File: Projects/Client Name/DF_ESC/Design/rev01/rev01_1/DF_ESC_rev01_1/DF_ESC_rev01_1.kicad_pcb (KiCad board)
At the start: 4 copper layers, 100 x 75 mm, 187 parts, among them J1 XT60PW-M, J2 HX25003-8AWB, J3 S6B-XH-SM4-TB(LF)(SN), J4 XH-3AWB, J5 7461084, J6 7461084, J7 7461084, J8 USB_C_Receptacle_USB2.0, Q1 HSBA15810C, Q2 HSBA15810C, Q3 HSBA15810C, Q4 HSBA15810C, Q5 HSBA15810C, Q6 HSBA15810C, SW1 SW_DIP_x01, U1 XH-2PWBPZ, U10 PUSB3AB6Z, U2 AMS1117-3.3, U3 STM32F405RGTx, U4 DRV8302DCAR, U5 S4B-XH-SM4-TB-(LF)(SN), U6 ESDCAN24-2BLY, U7 744227S, U8 SN65HVD230, U9 S6B-XH-SM4-TB(LF)(SN), Y1 Crystal_Small

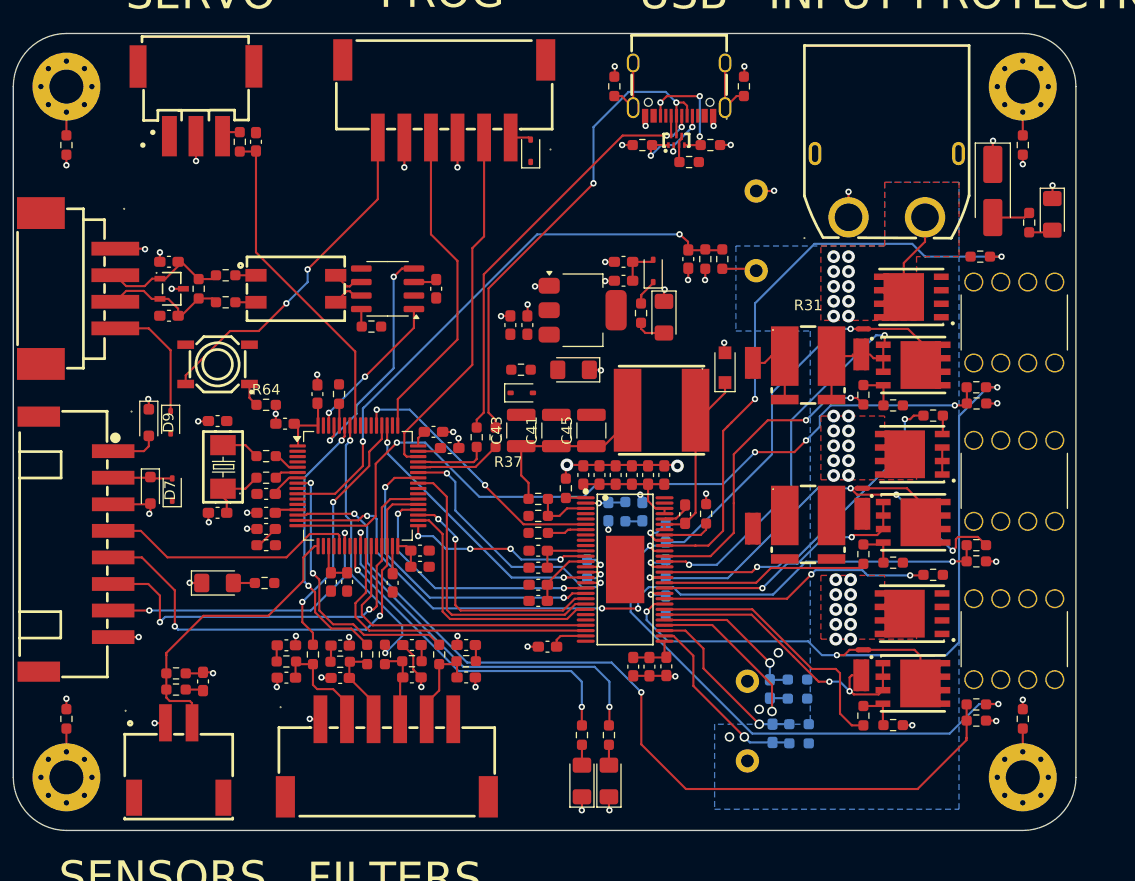
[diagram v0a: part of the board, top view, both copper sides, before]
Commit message: update 20240423
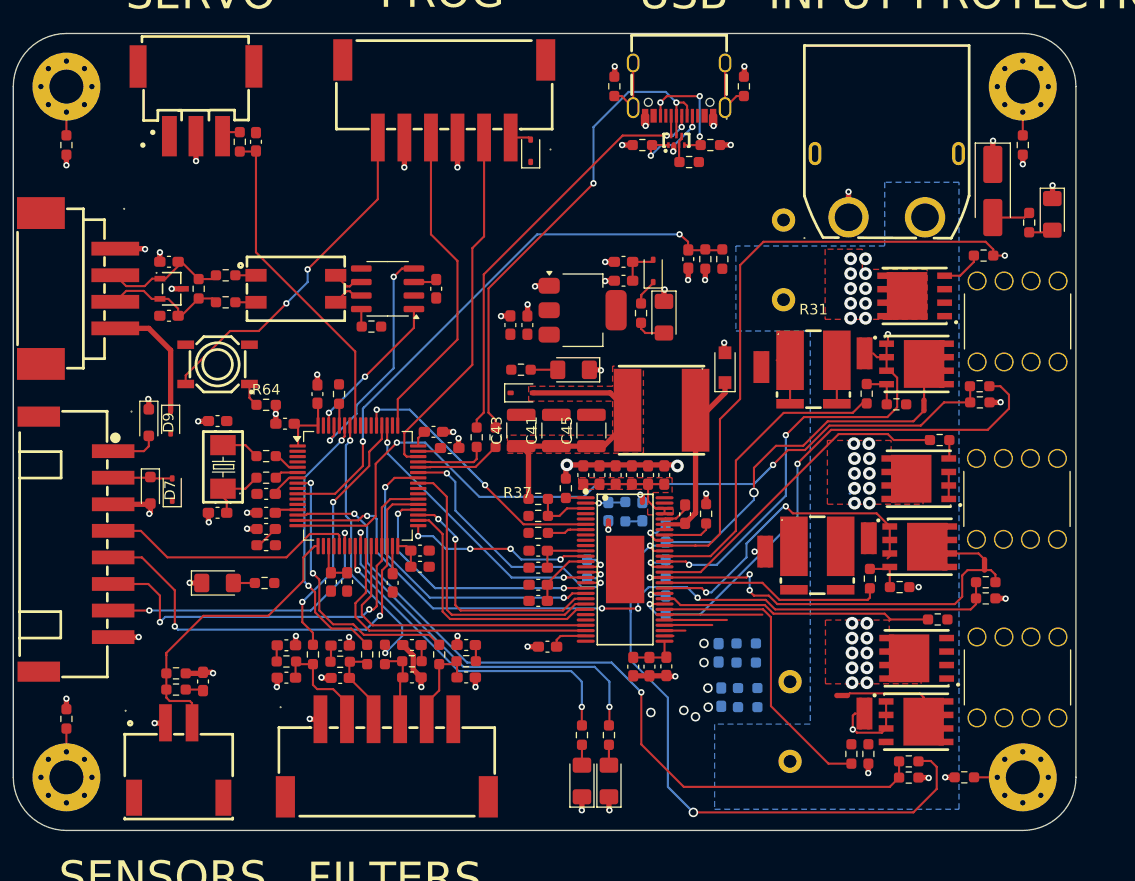
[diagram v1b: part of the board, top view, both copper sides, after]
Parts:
- moved NT4 13.6 mm to (275.2, 146.1), turned to -90 degrees
- moved NT1 9.18 mm to (269.5, 131.1), turned to -90 degrees
- moved R24 8.32 mm to (268.1, 164.6)
- moved R25 8.32 mm to (268.1, 166.1)
- moved R63 7.78 mm to (273.3, 166.1), turned to 180 degrees
- moved C48 5.91 mm to (250.2, 154.4)
- moved C49 5.91 mm to (250.4, 158.6)
- moved R29 5.91 mm to (252.8, 155.3)
- moved R28 5.91 mm to (252.8, 153.5)
- moved R34 5.91 mm to (252.9, 157.7)
- moved R35 5.91 mm to (252.9, 159.5)
- moved NT7 4.74 mm to (261.8, 158.4)
- moved Q5 4.22 mm to (268.8, 154.9)
- moved R39 4.22 mm to (270.8, 151.3)
- moved C1 4.01 mm to (257.0, 162.8)
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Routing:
- net H3_VS: track 72.6 -> 50.2 mm, vias 3 -> 2
- net S2_P: track 17.6 -> 0.84 mm
- net S2_N: track 16.5 -> 1.97 mm
- net S1_P: track 18.0 -> 4.50 mm
- net +VDC: track 31.4 -> 19.9 mm, vias 30 -> 31
- net H3_LOW: track 28.1 -> 16.9 mm, vias 2 -> 1
- net SENS3: track 83.9 -> 74.0 mm
- net /[5] - MOSFET DRIVER/+5V_DRV: track 17.3 -> 26.9 mm
- net H1_VS: track 81.9 -> 91.3 mm
- net S1_N: track 14.9 -> 5.87 mm
- net /[6] - MOSFETs/PHASE_1: track 7.60 -> 3.40 mm
- net /[6] - MOSFETs/PHASE_2: track 9.98 -> 6.05 mm
- net /[6] - MOSFETs/M_H1_RG: track 0.00 -> 3.89 mm
- net H2_LOW: track 25.5 -> 29.4 mm
- net Net-(Q6-G): track 3.97 -> 0.38 mm
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- added copper zone on F.Cu, net /[5] - MOSFET DRIVER/+5V_DRV
